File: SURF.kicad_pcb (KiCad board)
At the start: 4 copper layers, 33 x 30.7 mm, 30 parts, among them IC1 TPS7A0212PDBVR, IC2 TPS7A0228PDBVR, J1 Conn_01x10_Pin RIGHT, J2 Conn_01x10_Pin LEFT, J3 Conn_01x04, Q3 DMP3098LDM-7, U1 ESP32-S2-MINI-2

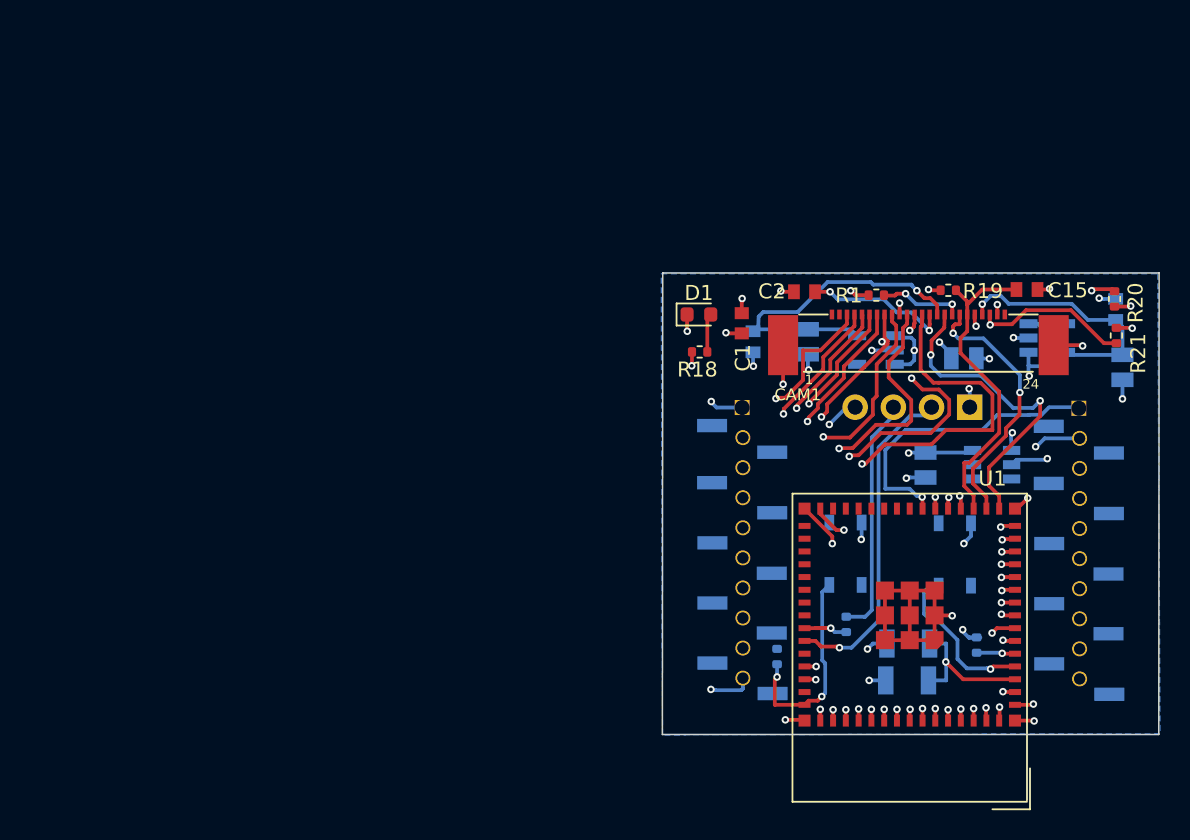
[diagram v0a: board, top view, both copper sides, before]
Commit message: new update
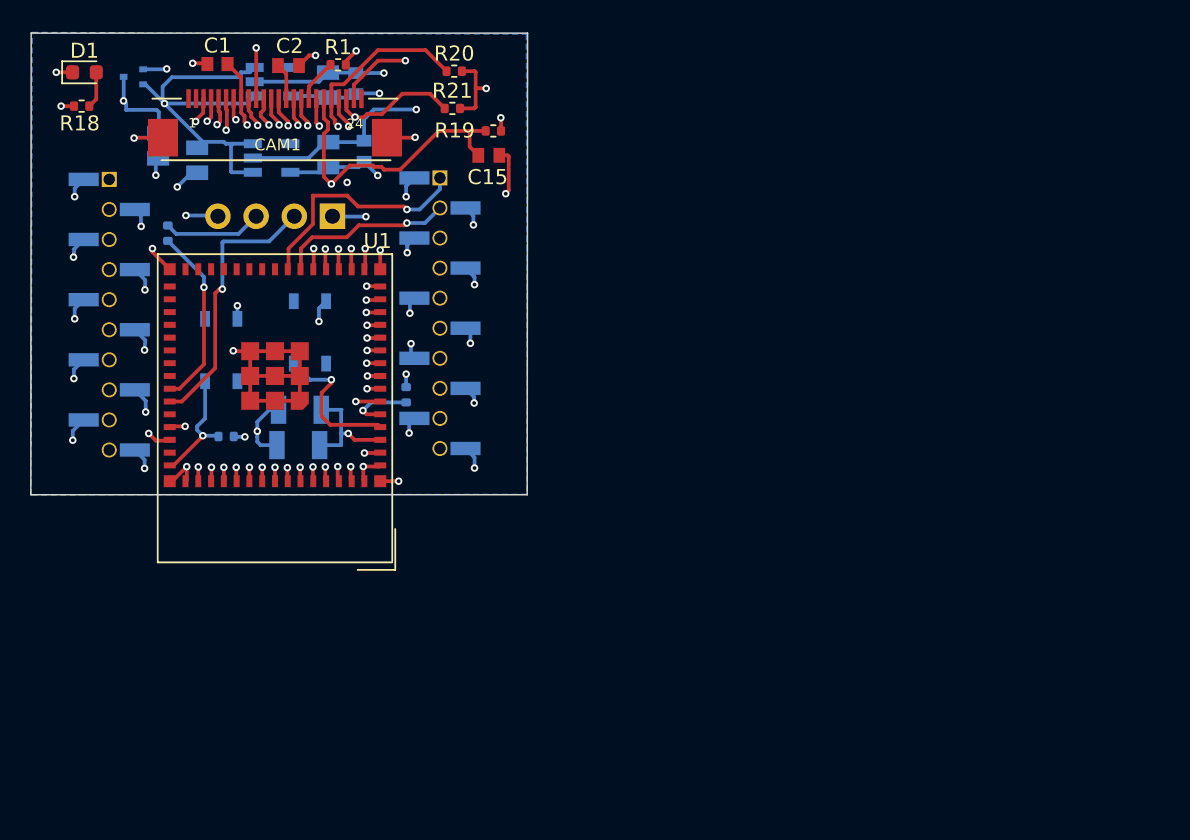
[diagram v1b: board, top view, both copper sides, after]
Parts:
- removed Q3: DMP3098LDM-7, DMP3098LDM-7:SOT95P285X140-6N
- added Q1: BSS84PWH6327XTSA1, Package_TO_SOT_SMD:SOT-523, B.Cu at (124.8, 57.9)
- CAM1: footprint OV2640:FPC-24 -> UPDATE_OV2640:ov2640-fcp_1
- J1, J2: footprint CONN_01X10_CRAZTFLIE:CONN_PINHEADERS_01X10_CRAZYFLIE -> UPDATE_CRAZYFLIE:CONN_PINHEADERS_01X10_CRAZYFLIE
- moved C19 56.1 mm to (137.8, 58.4), turned to 90 degrees
- moved C17 55.3 mm to (126.5, 62.4)
- moved IC2 54.2 mm to (134.2, 58.2)
- moved C20 52.7 mm to (139.6, 58.3)
- moved C18 52.7 mm to (129.1, 63.4), turned to -90 degrees
- moved R4 52.1 mm to (127.1, 68.2)
- moved R21 46.7 mm to (146.1, 60.0), turned to 0 degrees
- moved R20 46.5 mm to (146.2, 57.5), turned to 0 degrees
- moved BOOT1 45.4 mm to (136.6, 74.8)
- moved J1 45.2 mm to (141.4, 57.1)
- moved U1 45.1 mm to (134.2, 85.2)
- moved CAM1 44.9 mm to (134.5, 59.3)
- moved J2 44.8 mm to (119.4, 57.2)
- moved J3 44.3 mm to (138.1, 67.1)
- moved R18 44.2 mm to (121.4, 59.8)
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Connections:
- J1 pad 1: GND -> /GPIO18
- J1 pad 3: GND -> unconnected-(J1-Pin_3-Pad3)
- J1 pad 5: GND -> unconnected-(J1-Pin_5-Pad5)
- J1 pad 7: GND -> unconnected-(J1-Pin_7-Pad7)
- J1 pad 9: GND -> unconnected-(J1-Pin_9-Pad9)
- J2 pad 1: GND -> +3V0
- J2 pad 3: GND -> unconnected-(J2-Pin_3-Pad3)
- J2 pad 5: GND -> unconnected-(J2-Pin_5-Pad5)
- J2 pad 7: GND -> unconnected-(J2-Pin_7-Pad7)
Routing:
- net GND: track 75.0 -> 126.4 mm, vias 48 -> 59
- net /CAM_VCC: track 55.0 -> 29.0 mm, vias 6 -> 1
- net Net-(Q1-G): track 21.0 -> 44.6 mm
- net /GPIO13: track 17.6 -> 37.9 mm
- net /GPIO12: track 21.2 -> 40.8 mm
- net /GPIO2: track 40.1 -> 54.3 mm
- net /GPIO3: track 38.3 -> 51.4 mm
- net /GPIO14: track 21.2 -> 34.1 mm, vias 0 -> 2
- net /GPIO4: track 37.5 -> 49.1 mm
- net /GPIO5: track 36.7 -> 47.1 mm
- net Net-(J3-Pin_3): track 15.5 -> 6.59 mm
- net /TXD0: track 3.91 -> 12.2 mm
- net /GPIO6: track 35.9 -> 42.5 mm
- net /EN: track 14.1 -> 8.16 mm, vias 2 -> 1
- net +1V2: track 22.5 -> 16.8 mm, vias 1 -> 2
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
